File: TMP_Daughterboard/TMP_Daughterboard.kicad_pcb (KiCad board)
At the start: 2 copper layers, 1 part, among them U1 TMP1075NDRLR

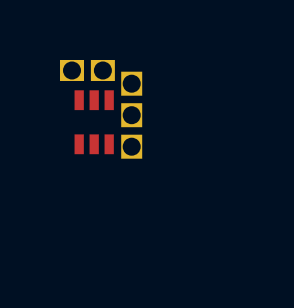
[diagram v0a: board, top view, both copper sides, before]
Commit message: daughter tmp board
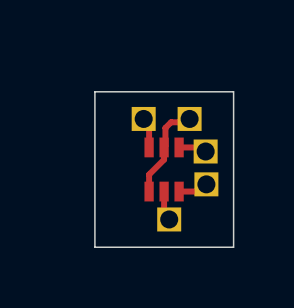
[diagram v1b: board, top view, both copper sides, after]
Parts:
- U1: footprint TMP_Daughterboard:TMP1075-MOD-A -> TMP_Daughterboard:TMP1075-MOD-B
- moved U1 2.85 mm to (152.4, 101.6)
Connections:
- U1 pad 2: unconnected-(U1-GND-Pad2) -> Net-(U1-A0)
- U1 pad 4: unconnected-(U1-A0-Pad4) -> Net-(U1-A0)
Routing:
- net Net-(U1-A0): track 0.00 -> 3.27 mm
- net unconnected-(U1-SDA-Pad6): track 0.00 -> 1.01 mm
- net unconnected-(U1-V+-Pad5): track 0.00 -> 1.00 mm
- net unconnected-(U1-ALERT-Pad3): track 0.00 -> 0.98 mm
- net unconnected-(U1-SCL-Pad1): track 0.00 -> 0.94 mm
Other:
- board outline added: 4.6 x 5.2 mm
